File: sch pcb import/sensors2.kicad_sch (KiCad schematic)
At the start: 32 parts, among them J501 Conn_Coaxial, J502 0734120114, J503 0734120114, J504 Micro_SD_Card, J505 Screw_Terminal_01x06, U501 RFM98W-433S2, U502 NEO-6M-GPS, U503 W25Q128JVS

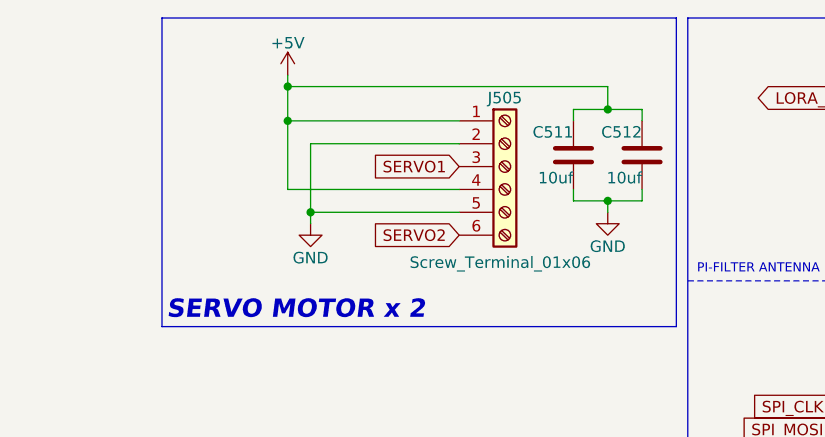
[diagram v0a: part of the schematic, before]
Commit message: rearranging for aesthetics
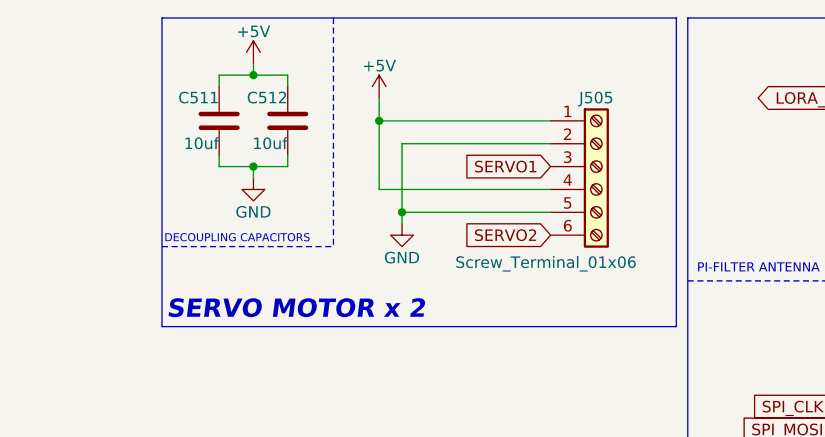
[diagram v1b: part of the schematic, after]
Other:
- moved on the sheet: C511, C512, J505
